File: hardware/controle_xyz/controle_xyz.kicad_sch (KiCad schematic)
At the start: 10 parts, among them Q1 TIP41, SW1 SW_Push, SW2 SW_Push, U1 PCF8574T

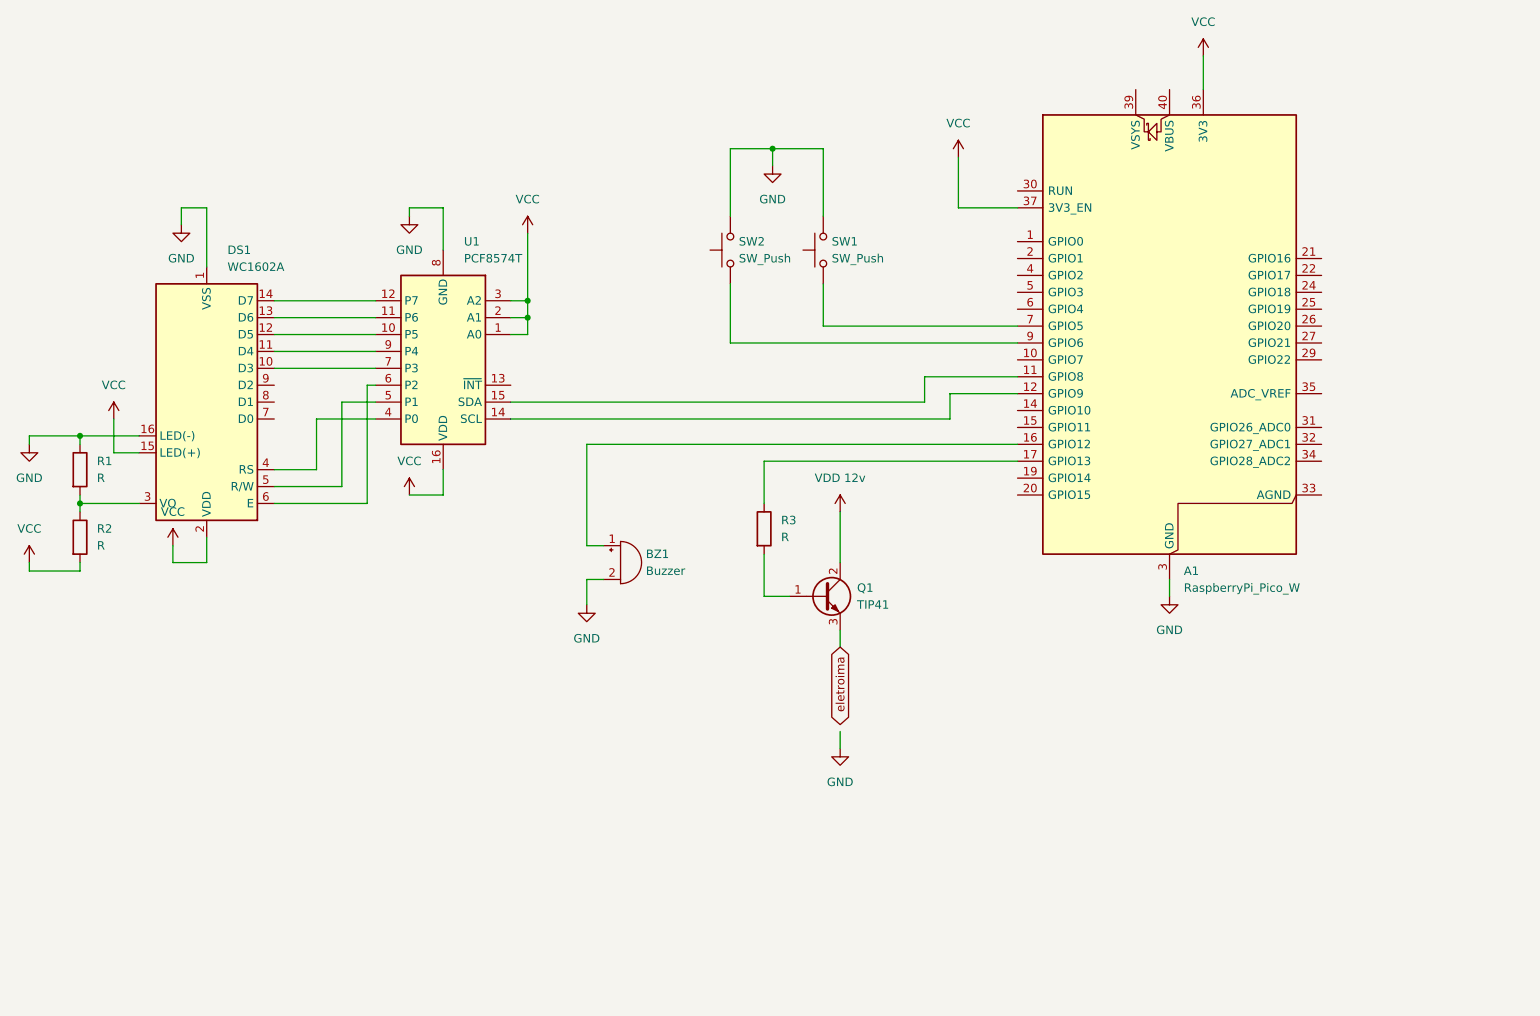
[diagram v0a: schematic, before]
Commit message: update hw sch
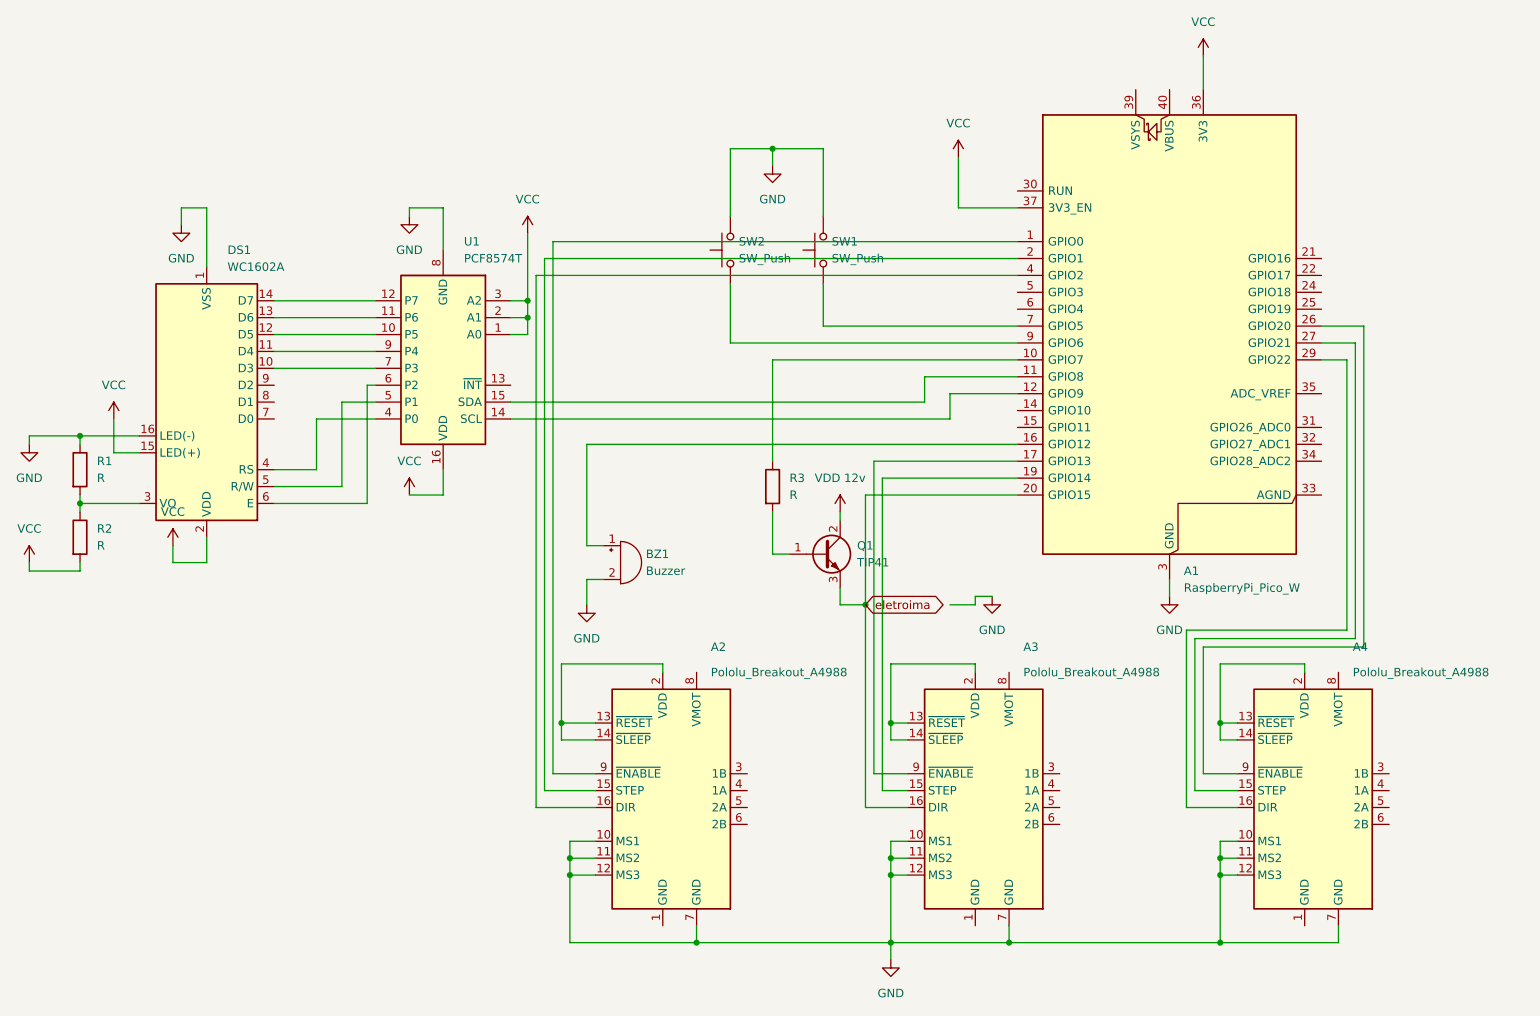
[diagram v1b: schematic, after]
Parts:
- added A2, A3, A4: Pololu_Breakout_A4988, Module:Pololu_Breakout-16_15.2x20.3mm, symbol Driver_Motor:Pololu_Breakout_A4988
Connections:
- net GND: now also A2.10 (MS1), A2.11 (MS2), A2.12 (MS3), A2.7 (GND), A3.10 (MS1), A3.11 (MS2), A3.12 (MS3), A3.7 (GND), A4.10 (MS1), A4.11 (MS2), A4.12 (MS3), A4.7 (GND)
- net eletroima: now also A1.20 (GPIO15), A3.16 (DIR)
- net at A1.1 (GPIO0): now also A2.9 (~{ENABLE})
- net at A1.10 (GPIO7): now also R3.1
- net at A1.17 (GPIO13): now also A3.9 (~{ENABLE}); no longer R3.1
- net at A1.19 (GPIO14): now also A3.15 (STEP)
- net at A1.2 (GPIO1): now also A2.15 (STEP)
- net at A1.26 (GPIO20): now also A4.9 (~{ENABLE})
- net at A1.27 (GPIO21): now also A4.15 (STEP)
- net at A1.29 (GPIO22): now also A4.16 (DIR)
- net at A1.4 (GPIO2): now also A2.16 (DIR)
- new net: A4.13 (~{RESET}), A4.14 (~{SLEEP}), A4.2 (VDD)
- new net: A3.13 (~{RESET}), A3.14 (~{SLEEP}), A3.2 (VDD)
- new net: A2.13 (~{RESET}), A2.14 (~{SLEEP}), A2.2 (VDD)
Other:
- moved on the sheet: Q1, R3
